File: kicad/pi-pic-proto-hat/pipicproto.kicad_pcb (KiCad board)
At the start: 2 copper layers, 65 x 56 mm, 33 parts, among them J1 Conn_01x02_Male, J10 Conn_01x13_Male, J2 Conn_01x02_Male, J22 Conn_01x13_Male, J3 Conn_01x02_Male, J4 Conn_01x02_Male, J5 Conn_01x02_Male, J6 Barrel_Jack_Switch, J7 Conn_01x20_Male, J8 Conn_01x06_Male, J9 Conn_01x06_Male, P1 Conn_02x20_Odd_Even, Q1 IRF4905, SW1 SW_Push, U1 PIC12F675-IP

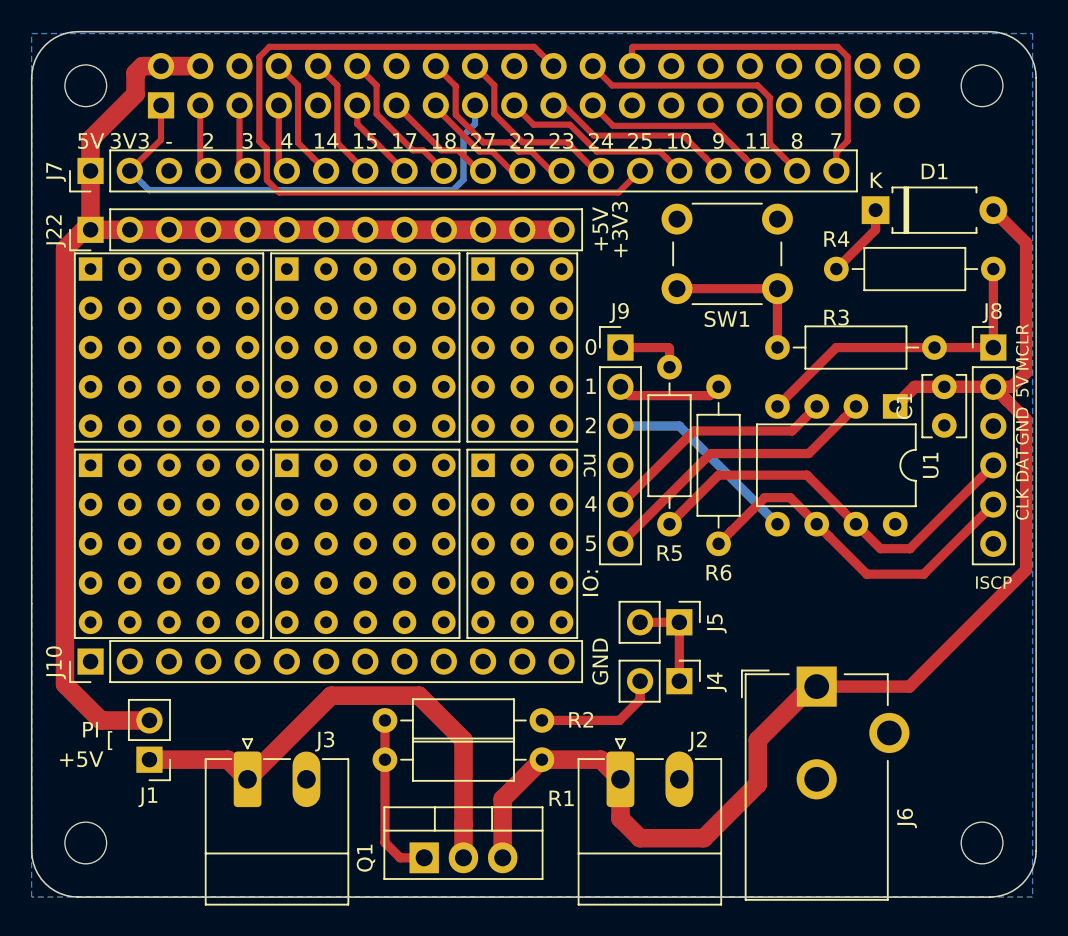
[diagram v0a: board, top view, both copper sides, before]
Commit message: version-e
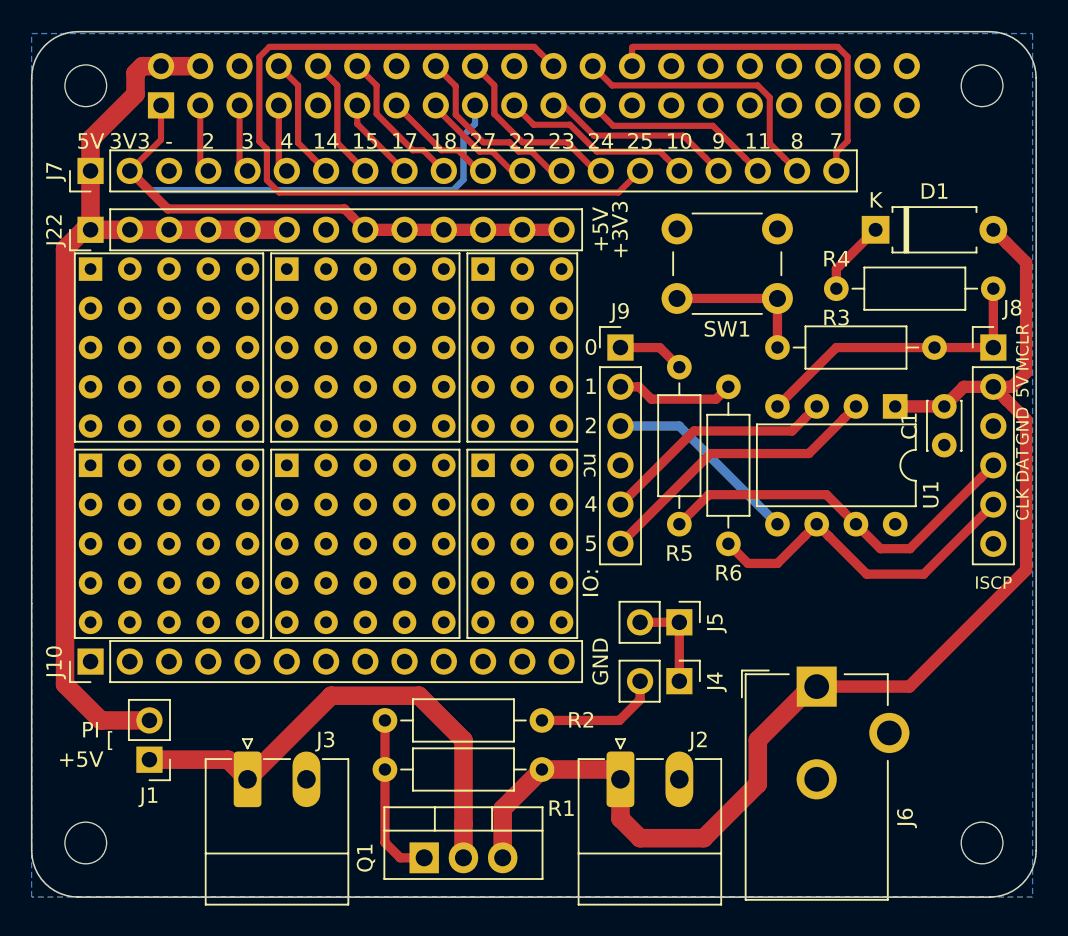
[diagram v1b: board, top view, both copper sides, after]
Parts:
- C1: footprint Capacitor_THT:C_Disc_D3.8mm_W2.6mm_P2.50mm -> Capacitor_THT:C_Disc_D3.0mm_W2.0mm_P2.50mm
- moved C1 1.27 mm to (259.1, 120.8)
- moved D1 1.27 mm to (254.6, 106.8)
- moved R4 1.27 mm to (262.2, 110.6)
- moved R6 0.64 mm to (245.1, 127.1)
- moved SW1 0.64 mm to (248.3, 111.3)
- moved R1 0.63 mm to (233.0, 141.7)
- moved R5 0.63 mm to (241.9, 125.9)
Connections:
- J22 pad 10: +5V -> +3V3
- J22 pad 11: +5V -> +3V3
- J22 pad 12: +5V -> +3V3
- J22 pad 13: +5V -> +3V3
- J22 pad 7: +5V -> Net-(J22-Pad7)
- J22 pad 8: +5V -> +3V3
- J22 pad 9: +5V -> +3V3
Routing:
- net +3V3: track 33.2 -> 62.7 mm
- net +5V: track 83.0 -> 65.2 mm
- net +5VP: track 84.7 -> 82.5 mm
- net /DAT: track 26.5 -> 24.8 mm
- net /MCLR: track 20.6 -> 19.4 mm
- net /CLK: track 22.9 -> 21.9 mm
- net /IO1: track 6.82 -> 7.65 mm
- net Net-(R3-Pad2): track 10.3 -> 9.67 mm
